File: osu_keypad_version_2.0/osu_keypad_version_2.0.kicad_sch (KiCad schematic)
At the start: 24 parts, among them SW1 SW_Push, U1 ATmega32U4-A, Y1 16Mhz

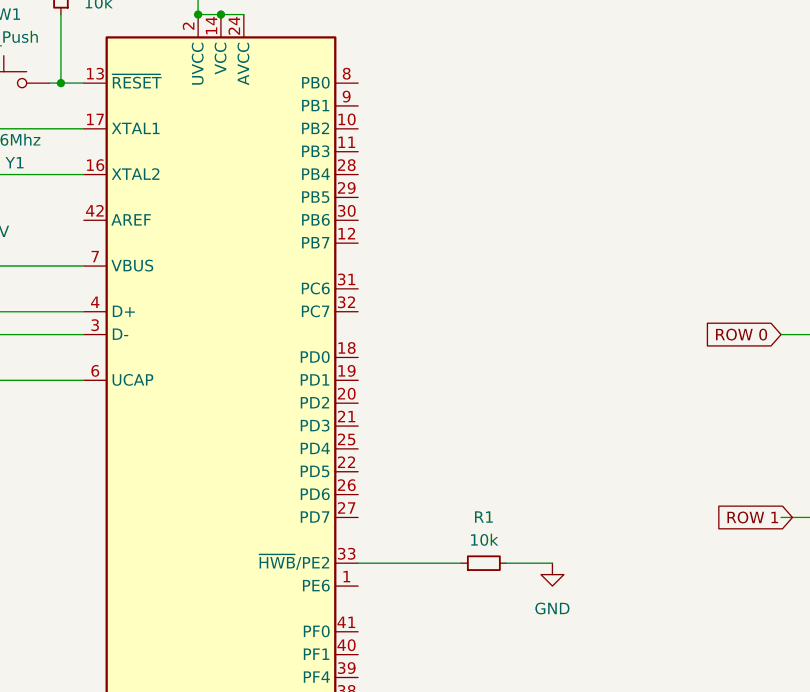
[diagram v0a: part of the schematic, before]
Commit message: routing done
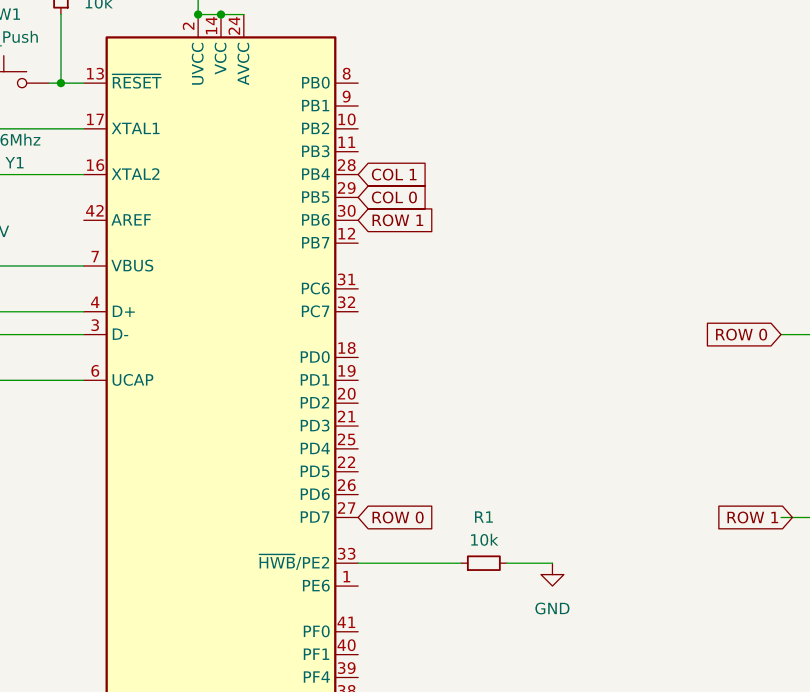
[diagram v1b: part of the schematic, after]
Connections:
- net COL 0: now also U1.29 (PB5)
- net COL 1: now also U1.28 (PB4)
- net ROW 0: now also U1.27 (PD7)
- net ROW 1: now also U1.30 (PB6)
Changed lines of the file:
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@@
+    )
+  )
+  (global_label "ROW 0" (shape input) (at 114.3 109.22 0) (fields_autoplaced)
+    (effects (font (size 1.27 1.27)) (justify left))
+    (property "Intersheetrefs" "${INTERSHEET_REFS}" (at 123.5142 109.22 0)
+      (effects (font (size 1.27 1.27)) (justify left) hide)
     )
   )
@@
       (effects (font (size 1.27 1.27)) (justify left) hide)
     )
+  )
+  (global_label "ROW 1" (shape input) (at 114.3 76.2 0) (fields_autoplaced)
+    (effects (font (size 1.27 1.27)) (justify left))
+    (property "Intersheetrefs" "${INTERSHEET_REFS}" (at 123.5142 76.2 0)
+      (effects (font (size 1.27 1.27)) (justify left) hide)
+    )
+  )
+  (global_label "COL 0" (shape input) (at 114.3 73.66 0) (fields_autoplaced)
+    (effects (font (size 1.27 1.27)) (justify left))
+    (property "Intersheetrefs" "${INTERSHEET_REFS}" (at 123.0909 73.66 0)
+      (effects (font (size 1.27 1.27)) (justify left) hide)
+    )
+  )
+  (global_label "COL 1" (shape input) (at 114.3 71.12 0) (fields_autoplaced)
+    (effects (font (size 1.27 1.27)) (justify left))
+    (property "Intersheetrefs" "${INTERSHEET_REFS}" (at 123.0909 71.12 0)
+      (effects (font (size 1.27 1.27)) (justify left) hide)
+    )
